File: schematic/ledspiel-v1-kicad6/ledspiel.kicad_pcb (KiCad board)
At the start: 2 copper layers, 90 x 56 mm, 160 parts, among them J1 Keys, J2 SWD Debug, J3 USART Debug, J5 USB_C_Receptacle_USB2.0, J70 Micro_SD_Card_Det, J80 Battery, Q10 BSS138, Q11 BSS138, Q12 BSS138, Q13 BSS138, Q14 BSS138, Q60 SFH300-3/4, Q70 IRLML6402, Q80 BSS138, Q81 IRLML6402, Q82 BSS138, U1 STM32F405RGTx, U100 LM4861, U2 USBLC6-2SC6, U60 TSOP382xx, U80 MCP1640CH, U81 LP38693MP-3.3, Y1 8MHz, Y2 32768Hz

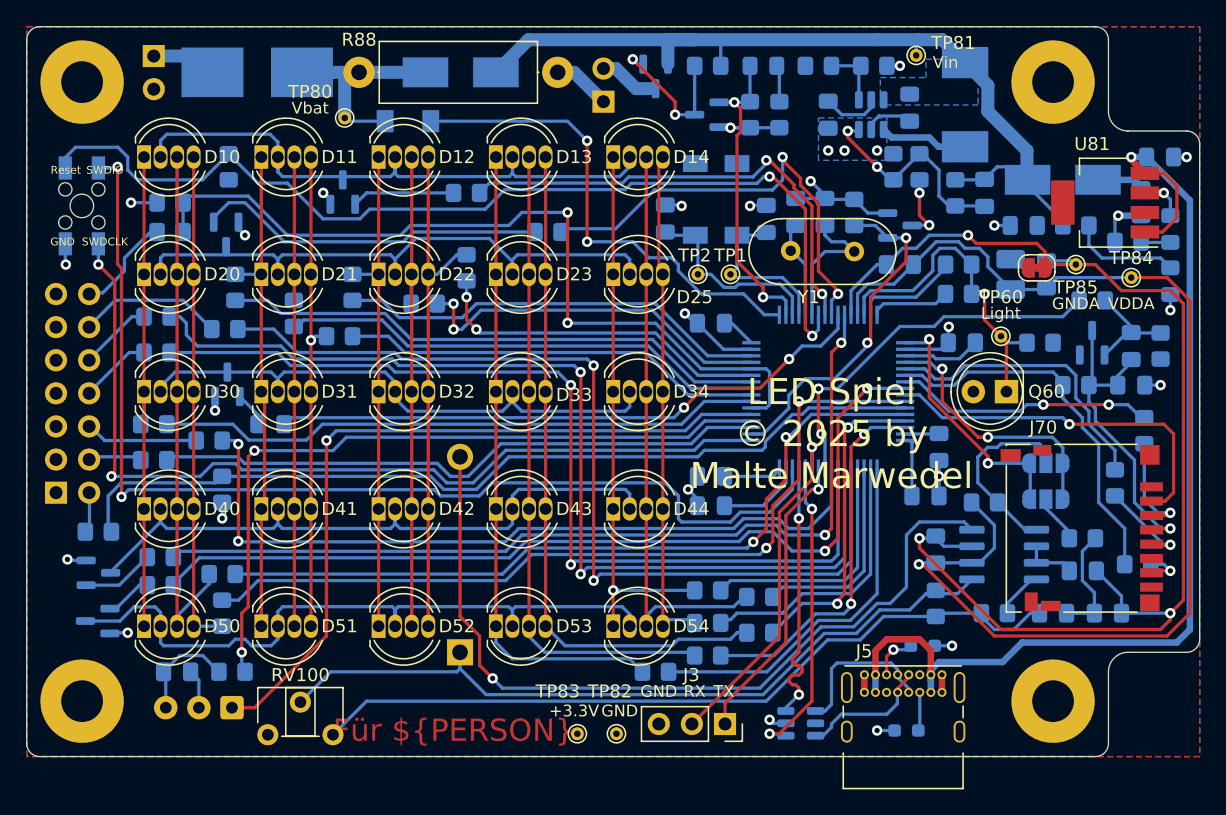
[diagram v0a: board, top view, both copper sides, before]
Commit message: WIP
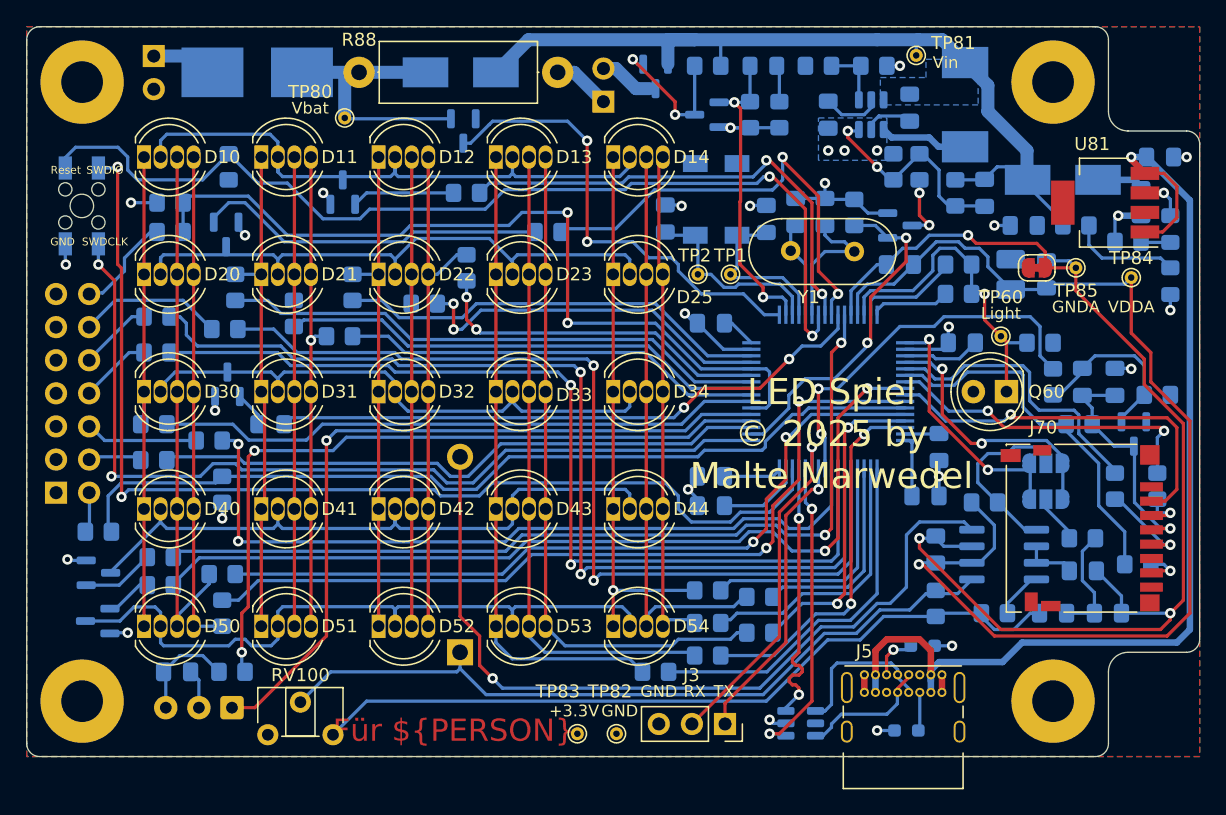
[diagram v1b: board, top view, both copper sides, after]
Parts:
- D84: value BAS32L -> BAT54C; footprint Diode_SMD:D_MiniMELF -> Package_TO_SOT_SMD:SOT-23
- R61: value 976kΩ -> 1MΩ
- R84: value 976kΩ -> 470kΩ
- R85: value 562kΩ -> 270kΩ
- moved Q70 7.70 mm to (184.9, 131.2), turned to -90 degrees
- moved R70 6.93 mm to (178.8, 127.2), turned to -90 degrees
- moved C71 4.65 mm to (181.0, 127.2)
- moved R73 4.37 mm to (186.8, 135.2)
- moved D84 4.32 mm to (133.5, 108.0), turned to -90 degrees
- moved R71 3.76 mm to (186.8, 128.2), turned to 0 degrees
- moved R72 3.01 mm to (180.8, 130.5)
- moved C70 1.27 mm to (183.5, 127.2), turned to 90 degrees
- moved R74 0.25 mm to (183.5, 135.2)
- moved TP85 0.25 mm to (180.5, 118.5)
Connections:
- D84 pad 1: Net-(D84-Pad1) -> /Vbat
- D84 pad 2: /Vbat -> unconnected-(D84-Pad2)
- U1 pad 1: Net-(D84-Pad1) -> Net-(U1-Pad1)
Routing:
- net Net-(D84-Pad1): track 37.6 -> 0.00 mm, vias 2 -> 0
- net Net-(U1-Pad1): track 0.00 -> 35.8 mm, vias 0 -> 2
- net Net-(C70-Pad1): track 24.3 -> 18.2 mm
- net /Spi1Mosi: track 19.7 -> 24.9 mm
- net Net-(C71-Pad1): track 8.32 -> 13.5 mm
- net /Vbat: track 16.2 -> 21.2 mm
- net Net-(J70-Pad3): track 8.22 -> 3.56 mm
- net GNDA: track 94.5 -> 91.1 mm
- net VDDA: track 90.2 -> 88.5 mm
- net /SdCs: track 28.3 -> 29.4 mm
- net /Spi1Miso: track 29.1 -> 28.5 mm
- net GND: track 68.1 -> 67.6 mm
- net Net-(JP100-Pad2): track 14.8 -> 14.3 mm

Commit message: Might be complete
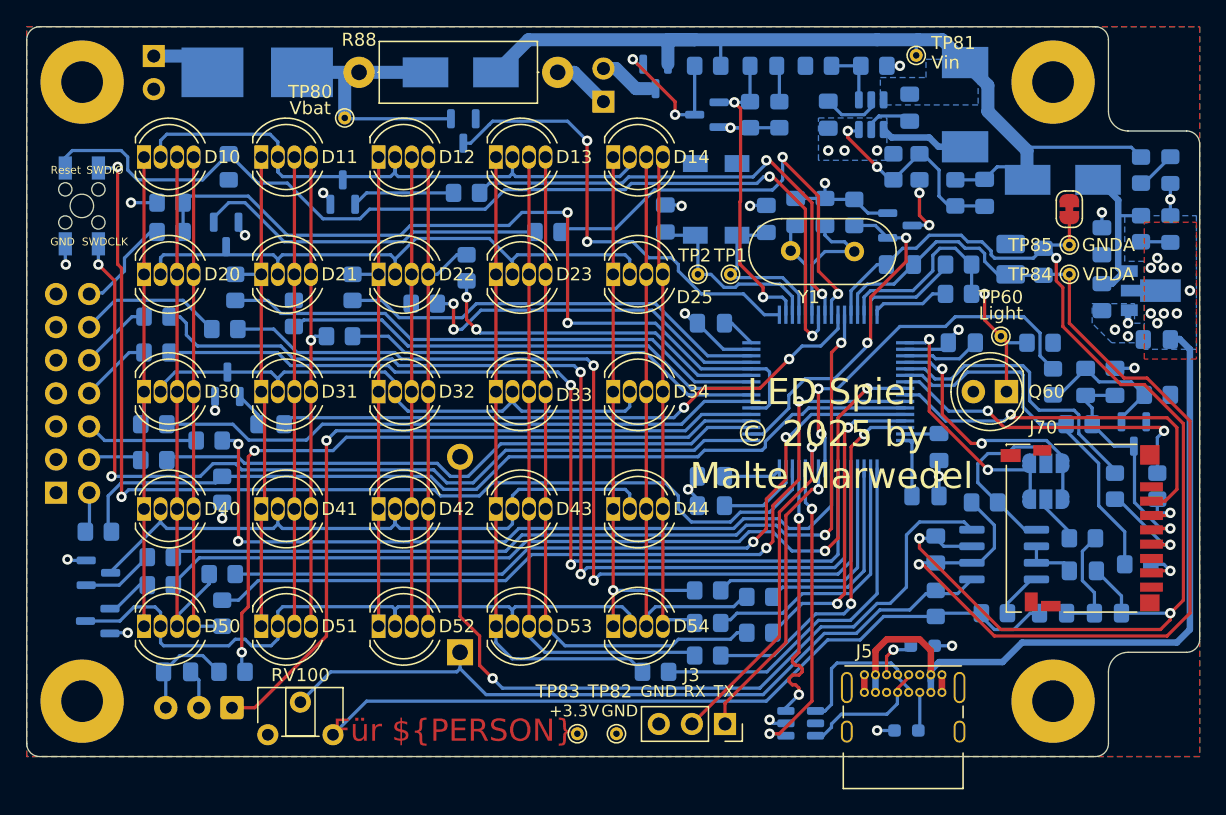
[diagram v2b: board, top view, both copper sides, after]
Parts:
- U81: value LP38693MP-3.3 -> MCP1703Ax-330xxMB; footprint Package_TO_SOT_SMD:SOT-223-5 -> Package_TO_SOT_SMD:SOT-89-3; moved to B.Cu
- moved C86 14.0 mm to (186.7, 124.0), turned to 180 degrees
- moved D81 8.53 mm to (187.8, 111.0)
- moved C87 7.88 mm to (182.5, 120.8)
- moved U81 7.60 mm to (186.2, 120.2), turned to 0 degrees
- moved R80 6.56 mm to (185.5, 111.0), turned to -90 degrees
- moved C83 6.12 mm to (182.5, 116.5), turned to 90 degrees
- moved JP80 5.15 mm to (180.0, 114.0), turned to -90 degrees
- moved TP84 4.76 mm to (180.0, 119.0)
- moved TP85 1.82 mm to (180.0, 116.8)
- moved R87 1.41 mm to (185.5, 115.5), turned to -90 degrees
- moved L2 1.16 mm to (175.5, 117.8)
- moved C84 0.99 mm to (178.0, 118.0)
- moved C71 0.25 mm to (181.2, 127.2)
- turned D83 to -90 degrees
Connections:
- D83 pad 1: Net-(D83-Pad1) -> GND
- D83 pad 2: Net-(C87-Pad1) -> Net-(D83-Pad2)
- R87 pad 1: Net-(D83-Pad1) -> Net-(C87-Pad1)
- R87 pad 2: GND -> Net-(D83-Pad2)
- U81 pad 1: /Vbus -> GND
- U81 pad 2: unconnected-(U81-Pad2) -> /Vbus
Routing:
- net /Vbus: track 82.1 -> 58.8 mm, vias 1 -> 9
- net Net-(D81-Pad2): track 8.47 -> 3.10 mm
- net /Vin: track 65.2 -> 69.7 mm
- net Net-(C87-Pad1): track 8.87 -> 12.6 mm, vias 1 -> 0
- net VDDA: track 88.5 -> 86.1 mm
- net Net-(C71-Pad1): track 13.5 -> 11.1 mm
- net Net-(D83-Pad2): track 0.00 -> 2.27 mm
- net Net-(D83-Pad1): track 2.27 -> 0.00 mm
- net GND: track 67.6 -> 65.5 mm, vias 28 -> 29
- net GNDA: track 91.1 -> 93.0 mm
- added copper zone on B.Cu, net /Vbus
- added copper zone on F.Cu, net /Vbus
